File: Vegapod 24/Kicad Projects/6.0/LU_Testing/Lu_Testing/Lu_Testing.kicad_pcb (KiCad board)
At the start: 2 copper layers, 179.5 x 87.4 mm, 132 parts, among them J1 DC Link, J2 17V-35V IN, J3 OUT, Q1 Q_NMOS_GDS, Q2 Q_NMOS_GDS, Q3 Q_PMOS_GSD, Q4 Q_PMOS_GSD, Q5 Q_PMOS_GSD, U1 KA78M05_TO252, U10 6N137, U11 ADUM4195-1BRIZ, U12 AMS1117-3.3, U13 B0505S-1WR3, U2 LM7815_TO220, U3 B0505S-1WR3, U4 IR2110, U5 LM324, U6 6N137, U7 6N137, U8 6N137, U9 STM32G474RET6

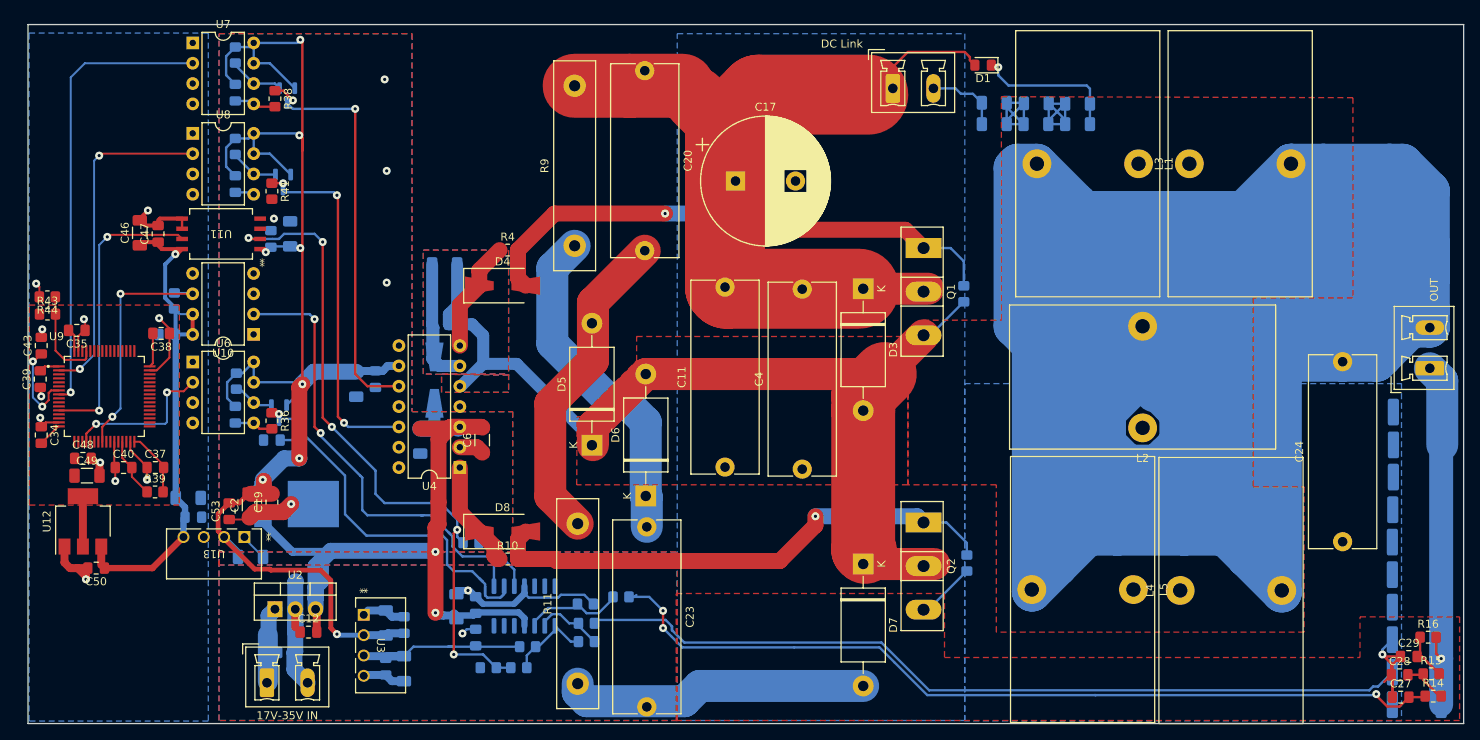
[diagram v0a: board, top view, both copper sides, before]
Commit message: LU Board Semi Final
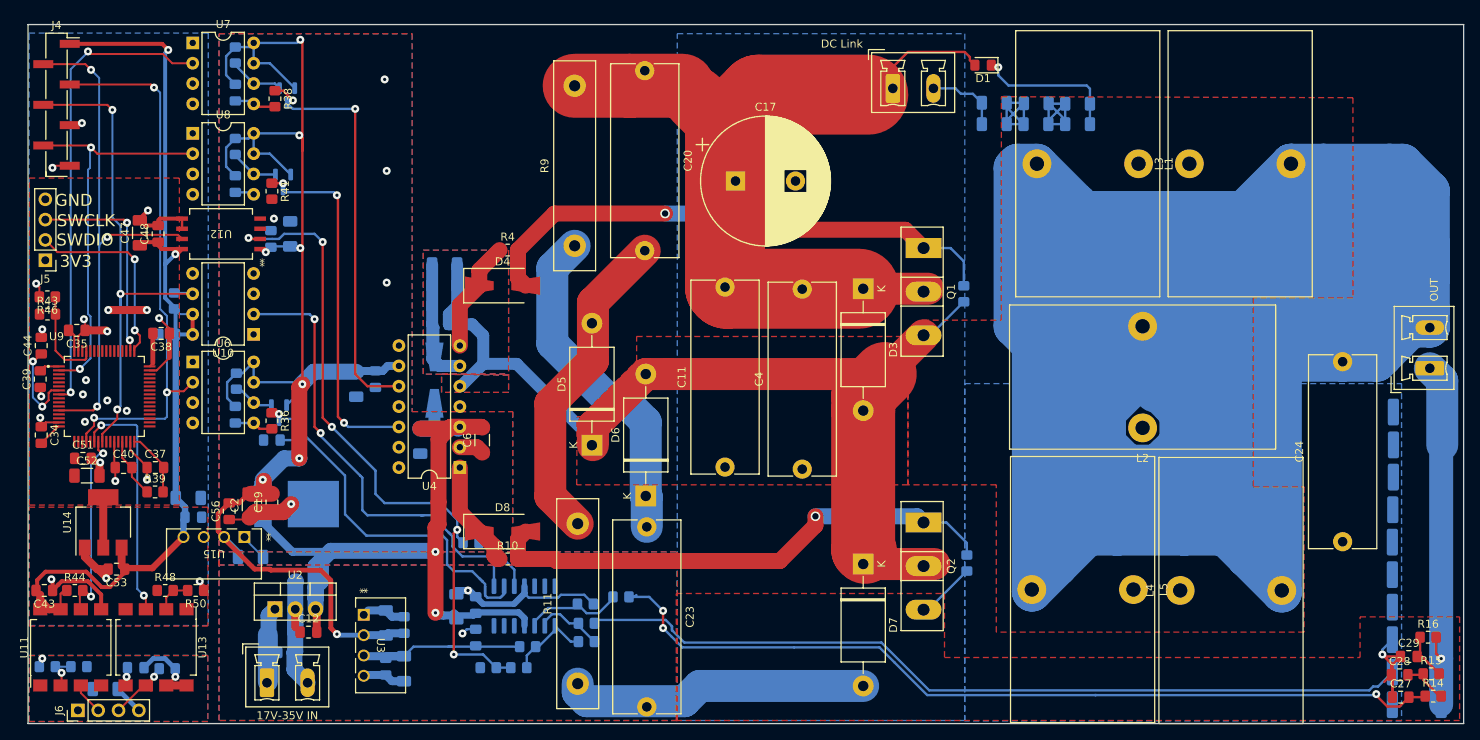
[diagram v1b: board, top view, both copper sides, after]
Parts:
- added C43: 100n, Capacitor_SMD:C_0805_2012Metric_Pad1.18x1.45mm_HandSolder, F.Cu at (79.1, 90.7)
- added C49: 10u, Capacitor_SMD:C_1206_3216Metric_Pad1.33x1.80mm_HandSolder, B.Cu at (86.7, 103.0)
- added C50: 100n, Capacitor_SMD:C_0805_2012Metric_Pad1.18x1.45mm_HandSolder, B.Cu at (90.6, 100.3)
- added J4: Conn_01x07_Male, Connector_PinHeader_2.54mm:PinHeader_1x07_P2.54mm_Vertical_SMD_Pin1Right, F.Cu at (80.6, 30.0)
- added J5: Conn_01x04_Male, Connector_PinHeader_2.54mm:PinHeader_1x04_P2.54mm_Vertical, F.Cu at (79.2, 49.4)
- added J6: Conn_01x04_Male, Connector_PinHeader_2.54mm:PinHeader_1x04_P2.54mm_Vertical, F.Cu at (83.3, 105.7)
- added R44: 470, Resistor_SMD:R_0805_2012Metric_Pad1.20x1.40mm_HandSolder, F.Cu at (82.9, 90.7)
- added R45: 470, Resistor_SMD:R_0805_2012Metric_Pad1.20x1.40mm_HandSolder, B.Cu at (79.5, 100.2)
- added R47: 470, Resistor_SMD:R_0805_2012Metric_Pad1.20x1.40mm_HandSolder, B.Cu at (83.4, 100.2)
- added R48: 470, Resistor_SMD:R_0805_2012Metric_Pad1.20x1.40mm_HandSolder, F.Cu at (94.2, 90.7)
- added R49: 470, Resistor_SMD:R_0805_2012Metric_Pad1.20x1.40mm_HandSolder, B.Cu at (94.5, 100.5)
- added R50: 470, Resistor_SMD:R_0805_2012Metric_Pad1.20x1.40mm_HandSolder, F.Cu at (98.0, 90.7)
- added U11: 6N137, Package_SO:SSO-8_6.7x9.8mm_P2.54mm_Clearance8mm, F.Cu at (82.4, 97.8)
- added U13: 6N137, Package_SO:SSO-8_6.7x9.8mm_P2.54mm_Clearance8mm, F.Cu at (93.1, 97.8)
- moved C53 2.54 mm to (88.1, 88.0)
- moved U14 2.54 mm to (86.5, 82.2)
- renumbered C43 to C44, C44 to C45, C45 to C46, C46 to C47, C47 to C48, C48 to C51, C49 to C52, C50 to C53, C51 to C54, C52 to C55, C53 to C56, C54 to C57, R44 to R46, U11 to U12, U12 to U14, U13 to U15
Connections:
- U9 pad 22: unconnected-(U9-Pad22) -> TXD
- U9 pad 23: unconnected-(U9-Pad23) -> RXD
- U9 pad 49: unconnected-(U9-Pad49) -> SWDIO
- U9 pad 50: unconnected-(U9-Pad50) -> SWCLK
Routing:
- net +5VD: track 65.3 -> 124.7 mm, vias 1 -> 2
- net DPWMADJ: track 19.2 -> 69.8 mm, vias 2 -> 3
- net DFB: track 30.8 -> 64.5 mm, vias 2 -> 3
- net TXD: track 0.00 -> 31.2 mm, vias 0 -> 2
- net DA0: track 36.8 -> 65.2 mm, vias 2 -> 3
- net SWCLK: track 0.00 -> 26.6 mm, vias 0 -> 2
- net RXD: track 0.00 -> 24.3 mm, vias 0 -> 2
- net SWDIO: track 0.00 -> 24.2 mm, vias 0 -> 2
- net GNDD: track 49.6 -> 70.8 mm, vias 11 -> 22
- net 5VCOMM: track 0.00 -> 15.1 mm, vias 0 -> 2
- net TXCOMM: track 0.00 -> 8.41 mm, vias 0 -> 1
- net DLIN: track 42.2 -> 50.3 mm
- net DHIN: track 56.9 -> 61.9 mm, vias 1 -> 3
- net Net-(R45-Pad1): track 0.00 -> 4.67 mm, vias 0 -> 1
- net Net-(R48-Pad2): track 0.00 -> 4.52 mm
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- added copper zone on F.Cu, net +5VD
- added copper zone on F.Cu, net 5VCOMM
- added copper zone on B.Cu, net GNDCOMM
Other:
- board text added: "3V3"
- board text added: "5V"
- board text added: "GND"
- board text added: "RX"
- board text added: "SWCLK"
- board text added: "SWDIO"
- board text added: "TX"
